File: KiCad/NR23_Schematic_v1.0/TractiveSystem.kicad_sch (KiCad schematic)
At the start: 32 parts, among them M1 Zero_7R_Motor

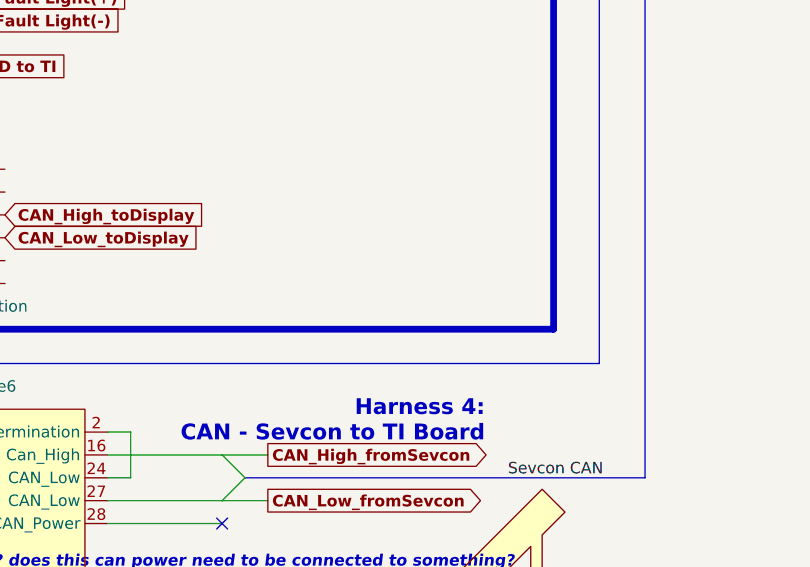
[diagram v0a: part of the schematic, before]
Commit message: end of day 05APR23
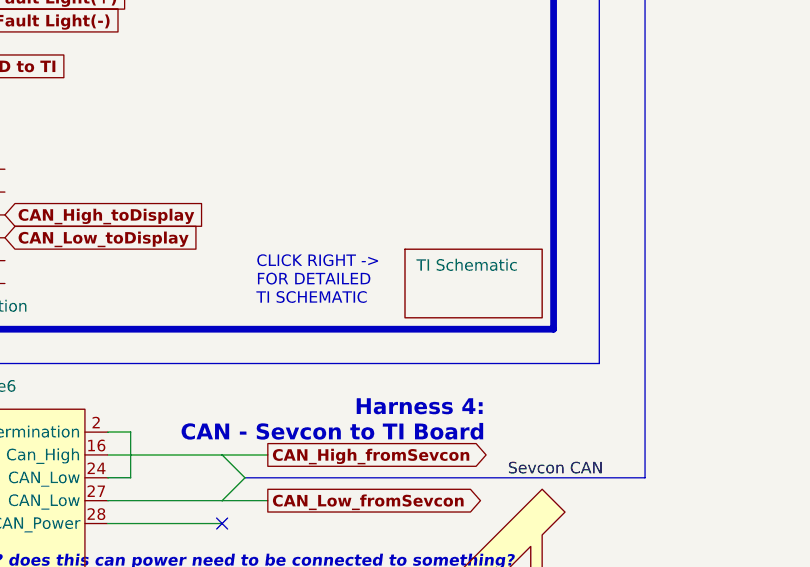
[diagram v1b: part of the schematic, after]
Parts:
- removed F?: Sevcon Fuse, symbol Device:Fuse
- removed J?: Deutsch, symbol Connector:Conn_01x04_Male
- removed K?: Key Switch Relay, Relay_THT:Relay_1P1T_NO_10x24x18.8mm_Panasonic_ADW11xxxxW_THT, symbol Relay:ADW11
- removed K?: Line Contactor, Relay_THT:Relay_1P1T_NO_10x24x18.8mm_Panasonic_ADW11xxxxW_THT, symbol Relay:ADW11
- removed SW?: HV Safety Switch (behind driver), symbol CamachosSymbols:Safety Switch
- removed U?: Throttle, symbol CamachosSymbols:Throttle
- removed U?: Sevcon_Gen4_Size6, symbol CamachosSymbols:Sevcon_Gen4_Size6
- added F?: Sevcon Fuse, symbol Device:Fuse
- added J?: Deutsch, symbol Connector:Conn_01x04_Male
- added K?: Line Contactor, Relay_THT:Relay_1P1T_NO_10x24x18.8mm_Panasonic_ADW11xxxxW_THT, symbol Relay:ADW11
- added K?: Key Switch Relay, Relay_THT:Relay_1P1T_NO_10x24x18.8mm_Panasonic_ADW11xxxxW_THT, symbol Relay:ADW11
- added SW?: HV Safety Switch (behind driver), symbol CamachosSymbols:Safety Switch
- added U?: Throttle, symbol CamachosSymbols:Throttle
- added U?: Sevcon_Gen4_Size6, symbol CamachosSymbols:Sevcon_Gen4_Size6
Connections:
- net CAN_High_fromSevcon: now also U?.16 (Can_High)
- net CAN_Low_fromSevcon: now also U?.27 (CAN_Low)
- net Cont1 Supply (+): now also K?.2
- net Line Contactor (Cont1): now also K?.1
- net at M1.1: now also U?. (M3)
- net at M1.2: now also U?. (M3)
- net at M1.3: now also U?. (M3)
- net at BTmain.(-), J?.5 (Pin_5): now also U?. (M3)
- net at J?.2 (Pin_2): now also U?. (M3)
- net at J?.3 (Pin_3): now also U?.15 (0_V)
- net at J?.4 (Pin_4): now also U?.19 (Digital_FS1)
- net at J?.1 (Pin_1): now also U?.21 (encoder_A)
- net at J?.3 (Pin_3): now also U?.22 (Pot1_WiperIn)
- net at J?.4 (Pin_4): now also U?.26 (+10V)
- net at J?.6 (Pin_6): now also U?.33 (Thermistor)
- net at J?.1 (Pin_1): now also U?.34 (Pot1_PwrSupply+)
- net at J?.2 (Pin_2): now also U?.35 (encoder_B)
- net at BTmain.(+): now also SW?.1 (A)
- net at J?.1 (Pin_1): now also K?.1
- net at J?.2 (Pin_2): now also K?.2
- net at SW?.2 (B): now also K?.3
- new net: J?.1 (Pin_1), U?.1 (pot_high_(red))
- new net: J?.2 (Pin_2), U?.2 (pot_low_(blk)), U?.4 (sw_o/p_(yl))
- new net: J?.3 (Pin_3), U?.3 (pot_wiper_(grn))
- new net: J?.4 (Pin_4), U?.5 (sw_i/p_(blu))
- new net: F?.1, U?. (M3)
- new net: F?.2, K?.4, U?. (M3)
- new net: K?.4, U?.1 (Key_Switch_In), U?.6 (Key_Switch_In)
- new net: U?.2 (CAN_Termination), U?.24 (CAN_Low)
- new net: K?.3, SW?.2 (B)
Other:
- added sheet TI Schematic (Microcontroller.kicad_sch)
- note added: "CLICK RIGHT -> FOR DETAILED TI SCHEMATIC"
